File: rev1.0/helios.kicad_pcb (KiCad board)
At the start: 4 copper layers, 17.8 x 33 mm, 61 parts, among them J1 USB_C_Receptacle_USB2.0, J2 helios-pinout, Q1 2N7002VC-, Q2 2N7002VC-, SW1 SWITCH, U1 USBLC6-2P6, U2 TLV75533PDQNR, U3 W25Q128JVPIQ, U4 RP2040, U5 74LVC1T45, Y1 12MHz

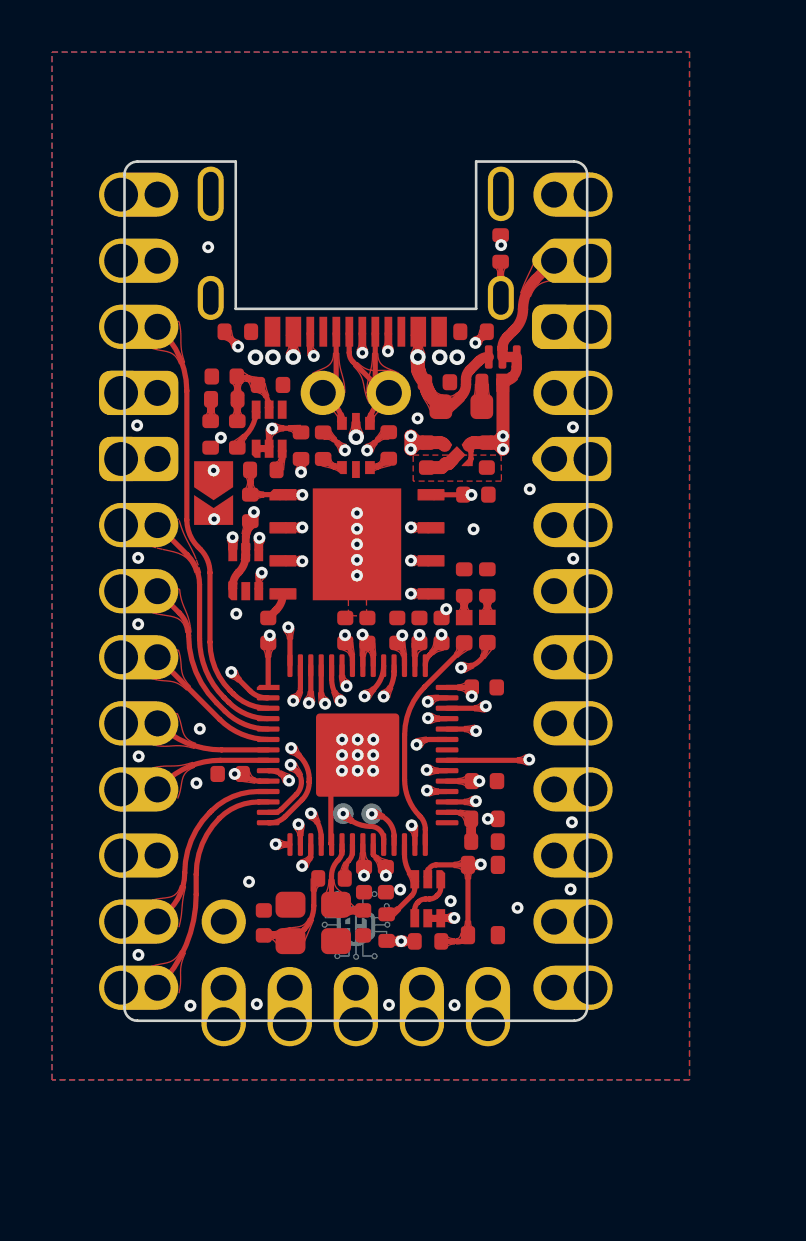
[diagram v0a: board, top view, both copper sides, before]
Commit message: manu change
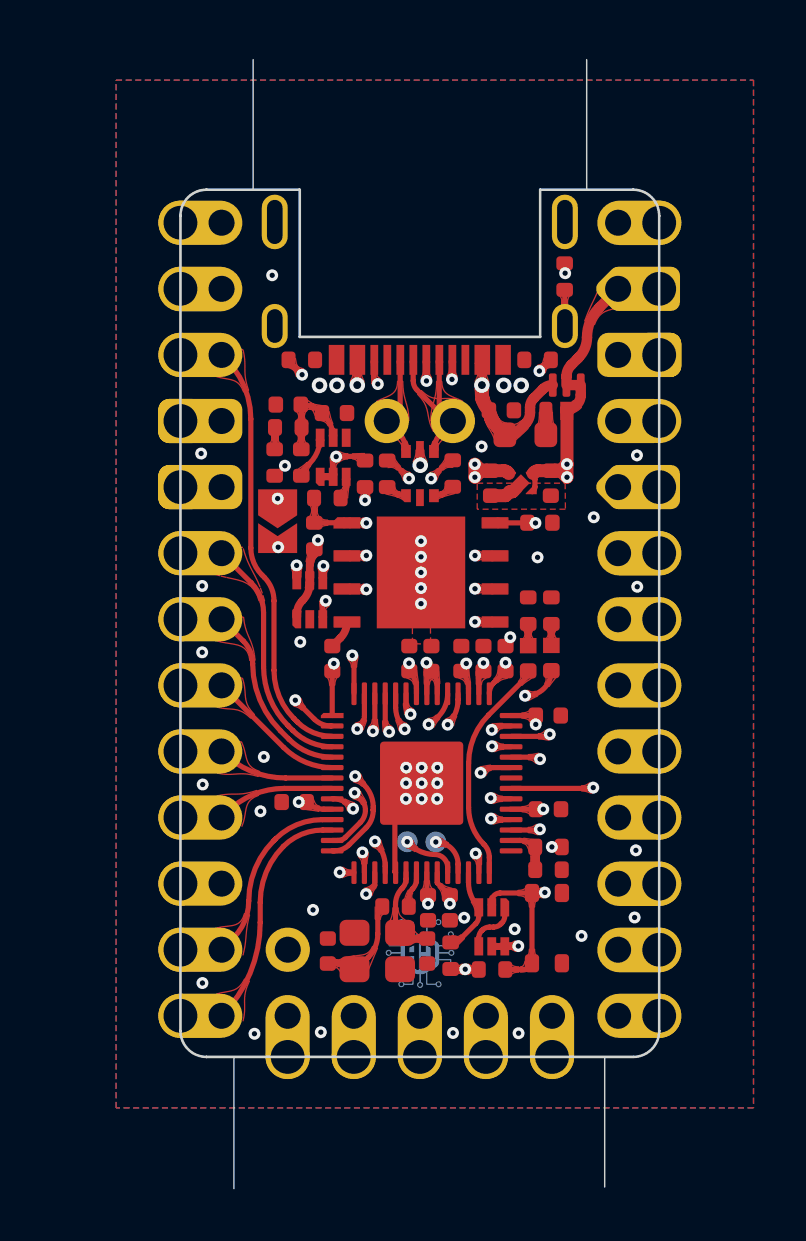
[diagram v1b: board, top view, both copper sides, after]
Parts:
- removed the REF** at (69.3, 81.3)
- removed the REF** at (82.6, 81.3)
- removed the REF** at (83.3, 115.3)
- removed the REF** at (68.6, 115.3)
- C1: value 4u7 -> 4.7u
- R12, R13: value 27R -> 27
- R16, R7, R8: value 5k1 -> 5.1k
- R4, R5, R6: value 51K -> 51k
- R9: value 1K -> 1k
- moved R10 2.69 mm to (83.5, 99.0)
- moved R15 2.69 mm to (82.6, 99.0)
- moved R7 2.69 mm to (82.9, 89.4)
- moved TP2 2.69 mm to (79.0, 107.9)
- moved C1 2.69 mm to (73.3, 91.1)
- moved C12 2.69 mm to (83.3, 106.7)
- moved C14 2.69 mm to (78.8, 100.9)
- moved C16 2.69 mm to (75.0, 100.9)
- moved C3 2.69 mm to (81.5, 91.3)
- moved C4 2.69 mm to (83.4, 94.1)
- moved C6 2.69 mm to (83.0, 95.7)
- moved C7 2.69 mm to (78.7, 112.1)
- moved C9 2.69 mm to (80.8, 100.9)
- moved D1 2.69 mm to (83.5, 100.9)
- moved D2 2.69 mm to (82.6, 100.9)
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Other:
- board size 17.8 x 33 mm -> 16.4 x 43.4 mm
